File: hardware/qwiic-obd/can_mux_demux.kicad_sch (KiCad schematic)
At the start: 12 parts, among them Q201 2N7002, Q202 2N7002, Q203 2N7002, U201 TS5A3359DCUR, U202 TS5A3359DCUR, U203 TS5A3359DCUR

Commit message: Added initial layout (parts dump)
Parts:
- U201, U202, U203: footprint DCU8 -> UltraLibrarian:TS5A3359DCUR
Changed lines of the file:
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@@
       (effects (font (size 1.524 1.524)))
     )
-    (property "Footprint" "DCU8" (id 2) (at 105.41 125.984 0)
+    (property "Footprint" "UltraLibrarian:TS5A3359DCUR" (id 2) (at 105.41 125.984 0)
       (effects (font (size 1.524 1.524)) hide)
     )
@@
       (effects (font (size 1.524 1.524)))
     )
-    (property "Footprint" "DCU8" (id 2) (at 104.14 89.154 0)
+    (property "Footprint" "UltraLibrarian:TS5A3359DCUR" (id 2) (at 104.14 89.154 0)
       (effects (font (size 1.524 1.524)) hide)
     )
@@
       (effects (font (size 1.524 1.524)))
     )
-    (property "Footprint" "DCU8" (id 2) (at 104.14 54.864 0)
+    (property "Footprint" "UltraLibrarian:TS5A3359DCUR" (id 2) (at 104.14 54.864 0)
       (effects (font (size 1.524 1.524)) hide)
     )

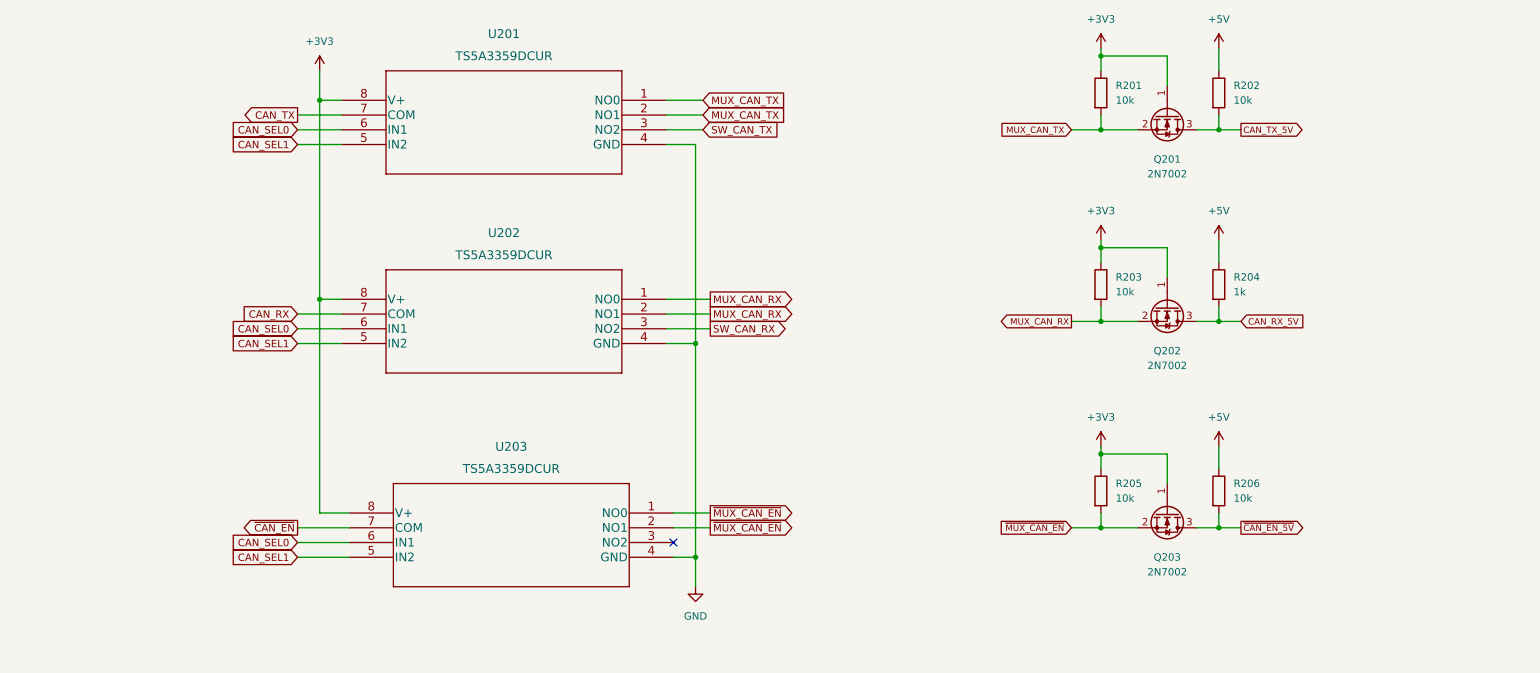
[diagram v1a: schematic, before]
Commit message: OK, layout v1 complete
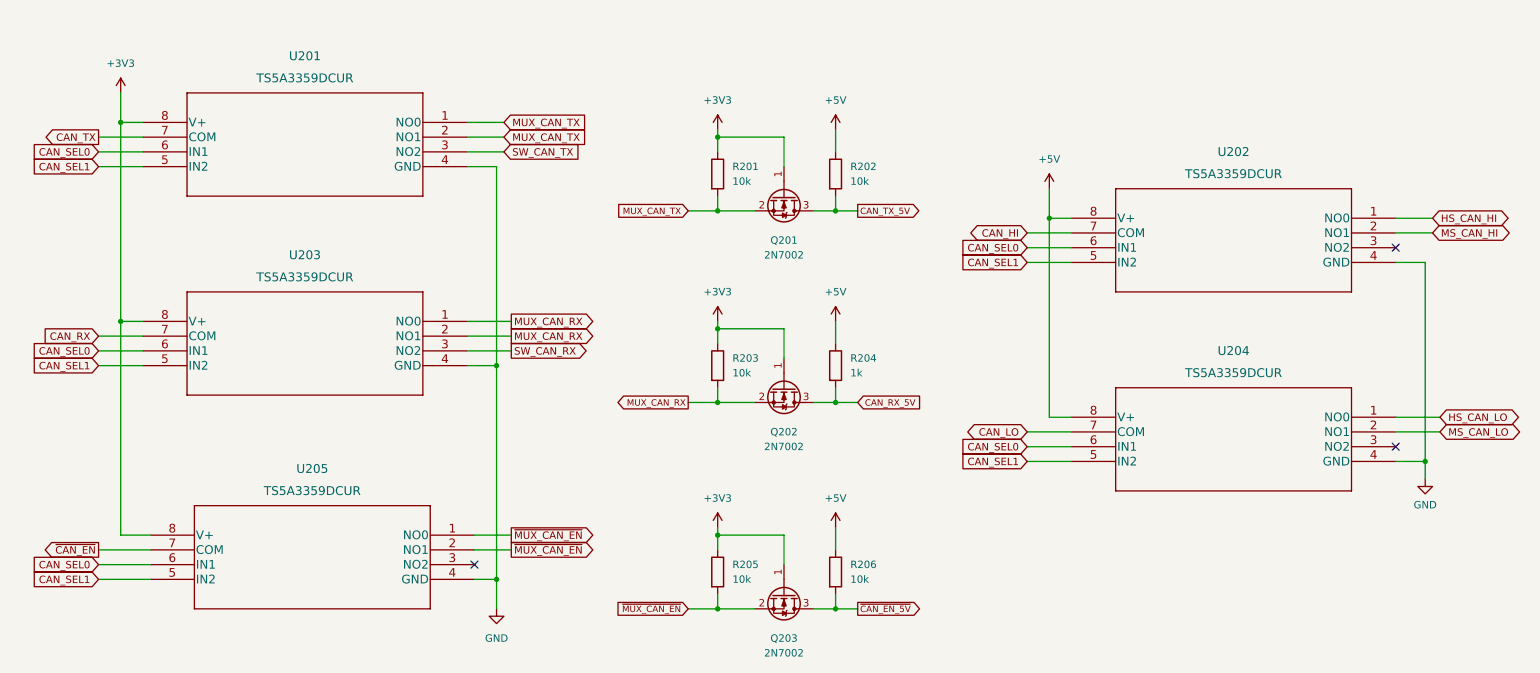
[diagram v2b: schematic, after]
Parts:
- added U202, U204: TS5A3359DCUR, UltraLibrarian:TS5A3359DCUR, symbol UltraLibrarian:TS5A3359DCUR
- renumbered U202 to U203, U203 to U205
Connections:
- net +5V: now also U202.8 (V+), U204.8 (V+)
- net CAN_SEL0: now also U202.6 (IN1), U204.6 (IN1)
- net CAN_SEL1: now also U202.5 (IN2), U204.5 (IN2)
- net GND: now also U202.4 (GND), U204.4 (GND)
- new net CAN_HI: U202.7 (COM)
- new net CAN_LO: U204.7 (COM)
- new net HS_CAN_HI: U202.1 (NO0)
- new net HS_CAN_LO: U204.1 (NO0)
- new net MS_CAN_HI: U202.2 (NO1)
- new net MS_CAN_LO: U204.2 (NO1)
- no-connect marks 1 -> 3
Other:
- moved on the sheet: Q201, Q202, Q203, R201, R202, R203, R204, R205, R206, U201, U203, U205
